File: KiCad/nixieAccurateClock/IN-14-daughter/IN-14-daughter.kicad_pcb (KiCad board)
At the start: 2 copper layers, 22.5 x 29.8 mm, 6 parts, among them J1 Conn_02x11_Top_Bottom, U1 HV509K6-G

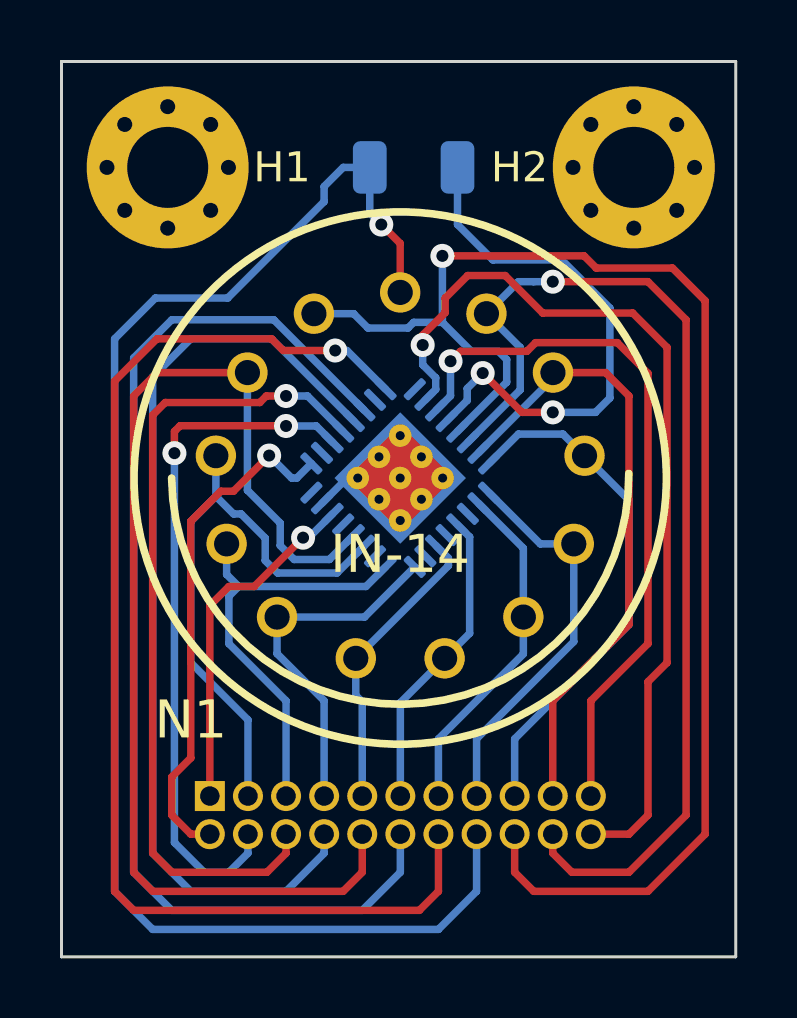
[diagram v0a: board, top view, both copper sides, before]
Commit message: WIP final feature push
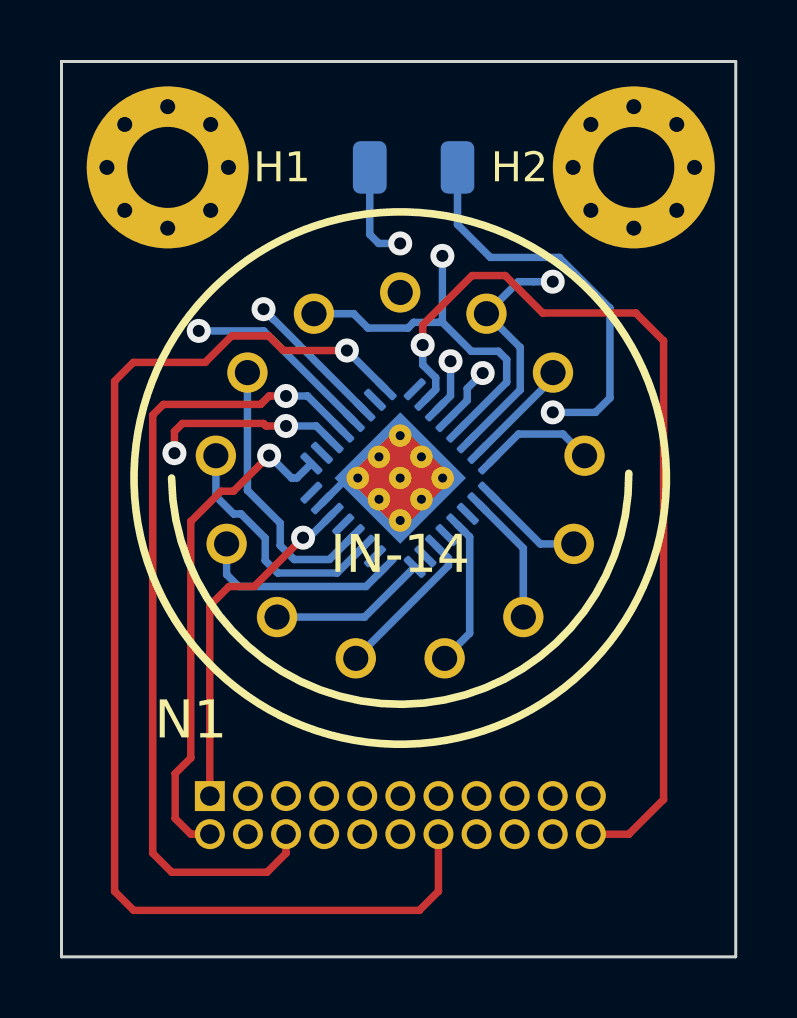
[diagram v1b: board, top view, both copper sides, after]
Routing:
- net /N_LHDP: track 48.3 -> 45.6 mm
- net /N_2: track 19.3 -> 20.7 mm
- net /N_3: track 14.7 -> 16.0 mm
- net /~{LATCH}: track 37.8 -> 38.6 mm, vias 0 -> 1
- net /~{POLARITY}: track 31.6 -> 31.9 mm, vias 0 -> 1
- added copper zone on In1.Cu, net GND
- added copper zone on In2.Cu, net GND
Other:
- copper layers 2 -> 4

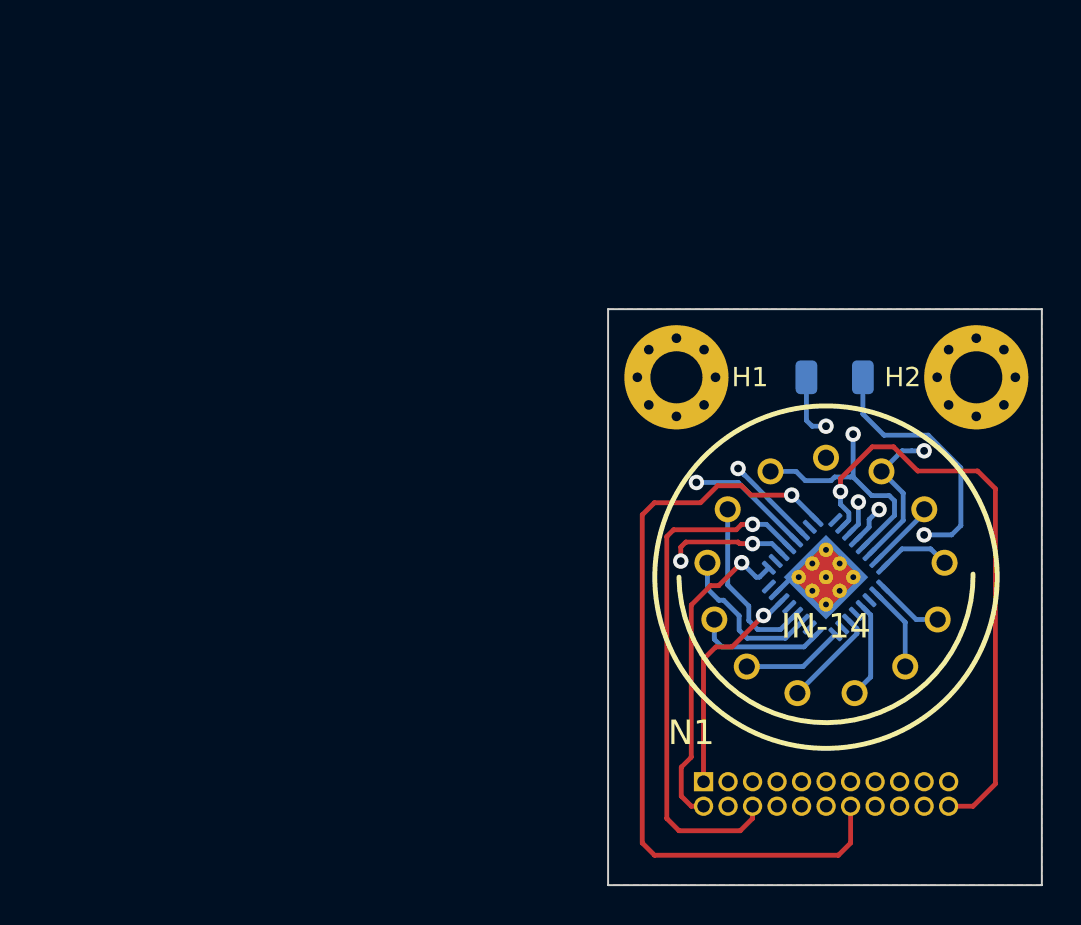
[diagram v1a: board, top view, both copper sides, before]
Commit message: reroute daughter board
Swapped standoffs and pin header orientation on IN-14 daughter board so that standoffs face outward.  This allows using the daughter board mounting for the mother board mounting.
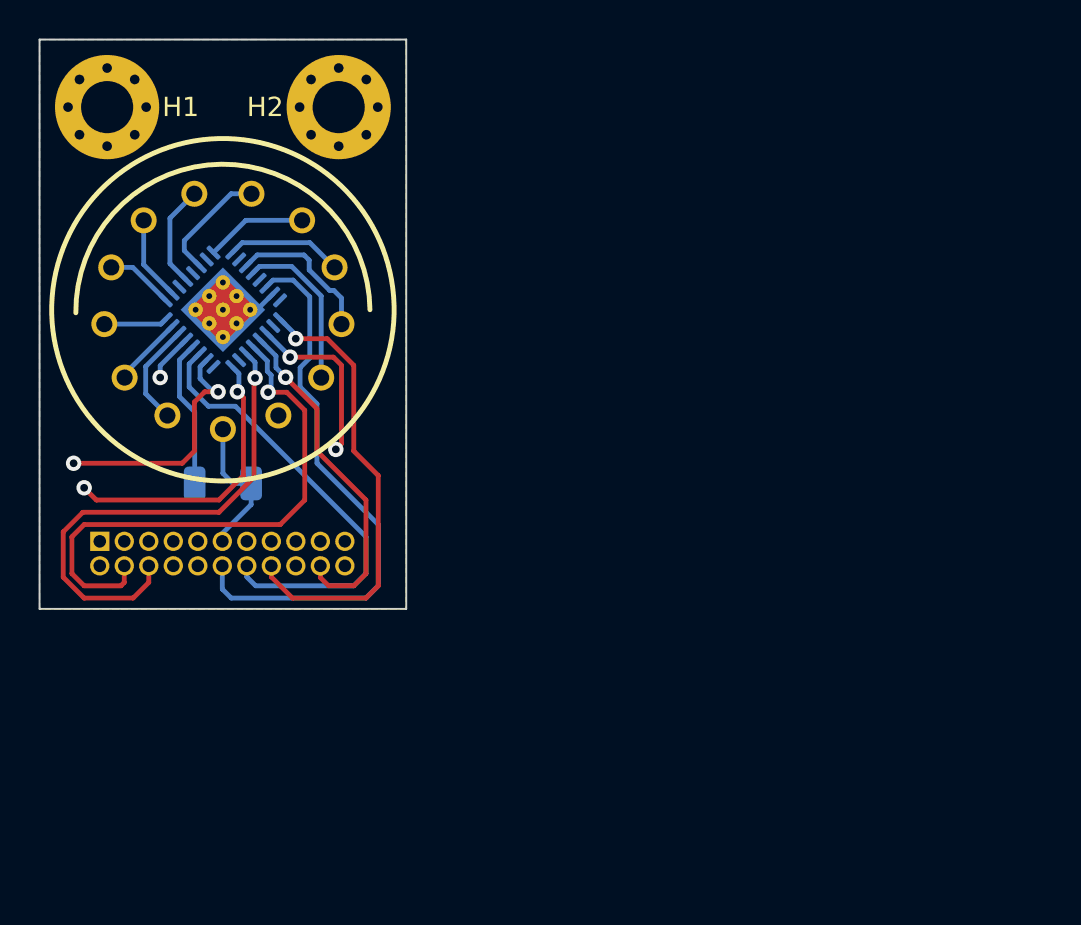
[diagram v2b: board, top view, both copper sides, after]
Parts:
- J1: value Conn_02x11_Top_Bottom -> Conn_02x11_Odd_Even
- moved H2 35.9 mm to (15.5, 3.50)
- moved N1 34.2 mm to (9.50, 14.0), turned to 0 degrees
- moved U1 34.2 mm to (9.50, 14.0), turned to -45 degrees
- moved J1 33.7 mm to (3.12, 26.0)
- moved H1 32.7 mm to (3.50, 3.50)
- moved R1 32.2 mm to (9.50, 23.0), turned to 0 degrees
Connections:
- J1 pad 1: VPP -> /N_7
- J1 pad 10: /N_1 -> +5V
- J1 pad 11: /N_6 -> /ANODE
- J1 pad 12: /~{LATCH} -> VPP
- J1 pad 13: /N_7 -> /N_LHDP
- J1 pad 14: /DOUT -> /HVGND
- J1 pad 15: /N_8 -> /N_1
- J1 pad 16: /ANODE -> /DIN
- J1 pad 17: /N_9 -> /N_2
- J1 pad 18: /N_LHDP -> /CLOCK
- J1 pad 19: /N_0 -> /N_3
- J1 pad 2: /DIN -> /N_6
- J1 pad 20: /N_RHDP -> +3.3V
- J1 pad 21: /HVGND -> /N_4
- J1 pad 22: +5V -> /N_5
- J1 pad 3: /N_2 -> /N_8
- J1 pad 4: /CLOCK -> /~{POLARITY}
- J1 pad 5: /N_3 -> /N_9
- J1 pad 6: +3.3V -> /~{LATCH}
- J1 pad 7: /N_4 -> /N_0
- J1 pad 8: /~{POLARITY} -> /DOUT
- J1 pad 9: /N_5 -> /N_RHDP
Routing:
- net /ANODE: track 49.3 -> 7.59 mm, vias 1 -> 0
- net /N_LHDP: track 45.6 -> 16.7 mm
- net /N_RHDP: track 35.7 -> 12.6 mm, vias 1 -> 0
- net /N_5: track 9.89 -> 32.6 mm
- net /N_6: track 10.2 -> 31.0 mm
- net /N_1: track 38.6 -> 18.1 mm
- net VPP: track 11.7 -> 29.4 mm, vias 1 -> 0
- net /DOUT: track 40.6 -> 26.1 mm, vias 1 -> 2
- net /N_4: track 11.9 -> 24.8 mm
- net /~{LATCH}: track 38.6 -> 26.1 mm
- net /N_7: track 11.6 -> 23.7 mm
- net /ANODE_DRIVE: track 18.2 -> 7.72 mm, vias 2 -> 0
- net +3.3V: track 27.3 -> 17.8 mm
- net /N_0: track 21.9 -> 13.2 mm
- net /DIN: track 16.9 -> 23.7 mm
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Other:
- board size 22.5 x 29.8 mm -> 19 x 29.5 mm
